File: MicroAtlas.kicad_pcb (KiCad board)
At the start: 4 copper layers, 20 x 32.8 mm, 38 parts, among them J1 TAGCONNECT, J2 Conn_01x02, J3 Conn_01x04_MountingPin, J4 SMA_Edgelaunch, J5 UFL, U1 NEO-F9P, U2 RAK3172-xx-43-SM-xI, U3 TPS7A2033PDBVR, U4 W25Q32JVZP, U5 TPS2116DRL, U6 LSM6DSV320XTR

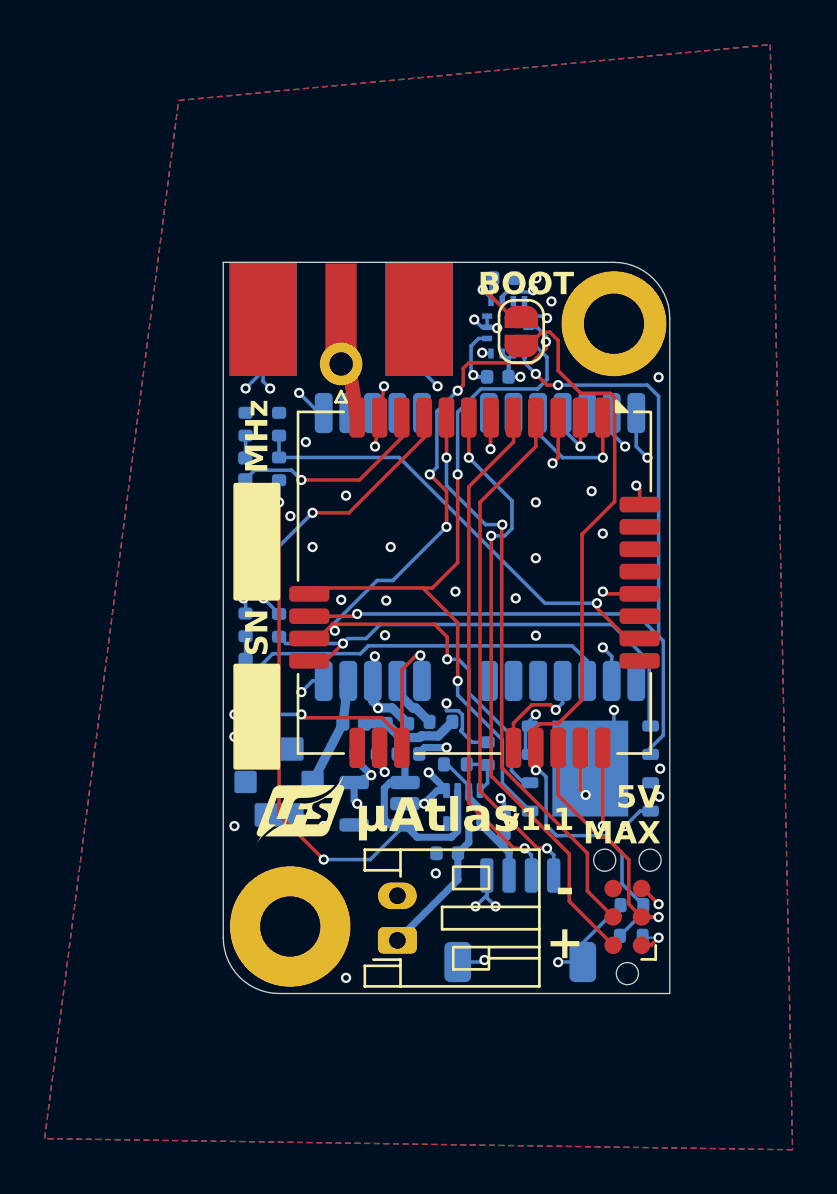
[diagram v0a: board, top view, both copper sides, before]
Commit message: prod v2.0
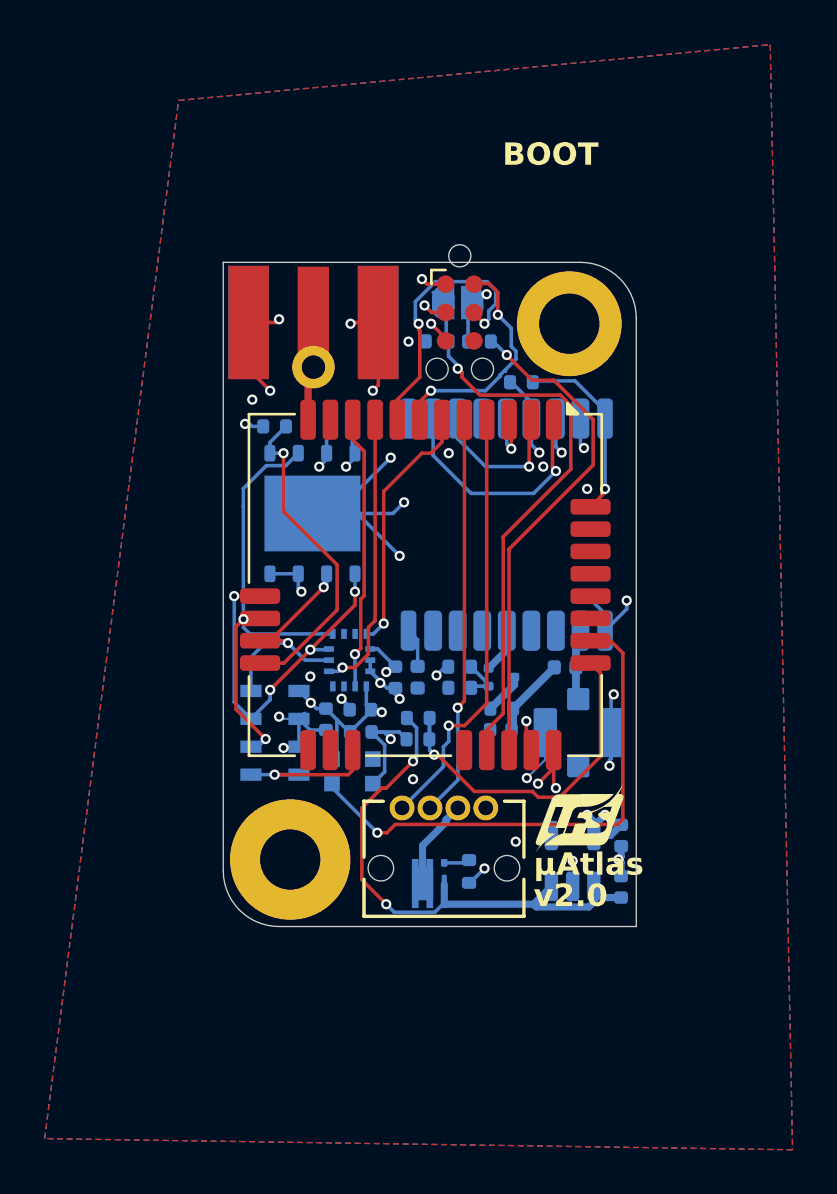
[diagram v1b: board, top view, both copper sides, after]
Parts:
- removed C46: 0.1uF, Capacitor_SMD:C_0402_1005Metric
- removed D7, D8: PPS, LED_SMD:LED_0402_1005Metric
- removed J3: Conn_01x04_MountingPin, Connector_JST:JST_SH_SM04B-SRSS-TB_1x04-1MP_P1.00mm_Horizontal
- removed R56, R57: 1k, Resistor_SMD:R_0402_1005Metric
- removed R58: 36k, Resistor_SMD:R_0402_1005Metric
- removed R59: 10k, Resistor_SMD:R_0402_1005Metric
- removed U4: W25Q32JVZP, Package_SON:WSON-8-1EP_6x5mm_P1.27mm_EP3.4x4.3mm
- added C48: 0.1uF, Capacitor_SMD:C_0402_1005Metric, B.Cu at (76.2, 52.8)
- added C51: 0.1uF, Capacitor_SMD:C_0402_1005Metric, B.Cu at (73.8, 41.6)
- added D1: WS2812B-2020, LED_SMD:LED_WS2812B-2020_PLCC4_2.0x2.0mm, B.Cu at (74.3, 57.0)
- added Q1: NTK3139PT1G, Package_TO_SOT_SMD:SOT-723, B.Cu at (81.0, 52.8)
- added Q2: SiA449DJ, Package_TO_SOT_SMD:Vishay_PowerPAK_SC70-6L_Single, B.Cu at (77.8, 62.1)
- added R49: 100k, Resistor_SMD:R_0402_1005Metric, B.Cu at (79.5, 61.5)
- added R60: 10k, Resistor_SMD:R_0402_1005Metric, B.Cu at (79.1, 52.4)
- added U7: LSM6DSV320XTR, PCM_SparkFun-Sensor:ST_LGA-14L_2.5x3.0mm_P0.5mm_4x3, B.Cu at (74.2, 52.1)
- C45: value 1uF -> 2.2uF
- C49, C50: value 4.7uF -> 0.1uF
- J2: value Conn_01x02 -> Conn_01x04_Socket; footprint Connector_JST:JST_PH_S2B-PH-K_1x02_P2.00mm_Horizontal -> FCU2025Lib:CONN_2200980000-SD_04P_MOL
- JP1: moved to B.Cu
- R55: value 1k -> 100R
- U1: value NEO-F9P -> W25Q32JVZP; footprint RF_GPS:ublox_NEO -> Package_SON:WSON-8-1EP_6x5mm_P1.27mm_EP3.4x4.3mm
- U3: value TPS7A2033PDBVR -> TPS7E7233
- U5: value TPS2116DRL -> MS5611-01BA; footprint Package_TO_SOT_SMD:SOT-583-8 -> Package_LGA:LGA-8_3x5mm_P1.25mm
- U6: value LSM6DSV320XTR -> MAX-M11S; footprint PCM_SparkFun-Sensor:ST_LGA-14L_2.5x3.0mm_P0.5mm_4x3 -> RF_GPS:ublox_MAX
- moved J1 28.1 mm to (79.1, 36.5), turned to -90 degrees
- moved R4 27.5 mm to (80.0, 37.8), turned to 180 degrees
- moved R3 26.7 mm to (78.1, 37.8)
- moved C47 20.4 mm to (74.6, 54.3), turned to 0 degrees
- moved R5 18.8 mm to (81.9, 39.6)
- moved R2 15.4 mm to (77.2, 55.6), turned to 180 degrees
- moved J5 13.6 mm to (84.4, 55.3), turned to 0 degrees
- moved R1 12.8 mm to (77.2, 54.7), turned to 0 degrees
- moved G*** 12.5 mm to (84.4, 59.2)
- moved C45 12.0 mm to (86.3, 59.9), turned to 90 degrees
- moved C44 11.2 mm to (86.3, 62.2), turned to -90 degrees
- moved R55 10.00 mm to (79.1, 53.3), turned to 0 degrees
- moved FB2 9.80 mm to (83.8, 52.4), turned to 180 degrees
- moved U5 9.07 mm to (70.8, 55.3), turned to 180 degrees
- moved U3 9.02 mm to (84.1, 61.1), turned to 90 degrees
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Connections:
- C49 pad 2: Net-(J2-Pin_1) -> +3V3
- C50 pad 2: +5V -> +3V3
- D6 pad 1: Net-(D6-K) -> GND
- J2 pad 1: Net-(J2-Pin_1) -> /TX
- J2 pad 2: GND -> /RX
- R54 pad 1: Net-(U1-VCC_RF) -> Net-(Q1-D)
- R55 pad 1: GND -> /EXT_ANT
- R55 pad 2: Net-(D6-K) -> Net-(Q1-G)
- U1 pad 1: unconnected-(U1-~{SAFEBOOT}-Pad1) -> /CS_FLASH
- U1 pad 2: +3V3 -> /MISO
- U1 pad 3: Net-(D6-A) -> +3V3
- U1 pad 4: /GPS_INT -> GND
- U1 pad 5: unconnected-(U1-USB_DM-Pad5) -> /MOSI
- U1 pad 6: unconnected-(U1-USB_DP-Pad6) -> /SCK
- U1 pad 7: unconnected-(U1-VDD_USB-Pad7) -> +3V3
- U1 pad 8: /GPS_NRST -> +3V3
- U1 pad 9: Net-(U1-VCC_RF) -> GND
- U2 pad 10: /P2 -> /IMU_INT2
- U2 pad 19: /GPS_NRST -> /CS_BARO
- U2 pad 20: /GPS_INT -> unconnected-(U2-PA9-Pad20)
- U2 pad 25: unconnected-(U2-PA10/PIN_A3-Pad25) -> /VDIV
- U2 pad 26: /VDIV -> /RGB
- U2 pad 3: /IMU_INT2 -> /GPS_INT
- U2 pad 32: /IMU_CS -> /GPS_NRST
- U2 pad 9: /P1 -> /IMU_CS
- U5 pad 1: GND -> +3V3
- U5 pad 2: V_LIPO -> GND
- U5 pad 3: +5V -> GND
- U5 pad 4: Net-(U5-PR1) -> /CS_BARO
- U5 pad 5: +5V -> /CS_BARO
- U5 pad 6: Net-(J2-Pin_1) -> /MISO
- U5 pad 7: V_LIPO -> /MOSI
- U5 pad 8: unconnected-(U5-ST-Pad8) -> /SCK
- U6 pad 1: /MISO -> GND
- U6 pad 10: unconnected-(U6-OCS_Aux-Pad10) -> GND
- U6 pad 11: unconnected-(U6-SDO_Aux-Pad11) -> Net-(J5-In)
- U6 pad 12: /IMU_CS -> GND
- U6 pad 13: /SCK -> unconnected-(U6-LNA_EN-Pad13)
- U6 pad 14: /MOSI -> Net-(Q1-S)
- U6 pad 2: GND -> /GPS_RX
- U6 pad 3: GND -> /GPS_TX
- U6 pad 4: /IMU_INT1 -> /TP
- U6 pad 5: +3V3 -> /GPS_INT
- U6 pad 6: GND -> +3V3
- U6 pad 7: GND -> +3V3
- U6 pad 9: /IMU_INT2 -> /GPS_NRST
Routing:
- net /SCK: track 36.0 -> 11.4 mm, vias 6 -> 2
- net /RGB: track 0.00 -> 23.4 mm, vias 0 -> 1
- net /MISO: track 39.6 -> 21.1 mm, vias 3 -> 2
- net /SWDIO: track 27.4 -> 10.5 mm
- net /MOSI: track 32.5 -> 16.2 mm, vias 2 -> 4
- net /NRST: track 12.1 -> 28.0 mm, vias 1 -> 2
- net Net-(D6-A): track 17.1 -> 2.03 mm
- net /SWCLK: track 25.9 -> 12.3 mm
- net /P1: track 11.5 -> 0.00 mm, vias 1 -> 0
- net /P2: track 9.06 -> 0.00 mm, vias 1 -> 0
- net /BOOT: track 34.9 -> 26.8 mm
- net /CS_FLASH: track 22.6 -> 14.6 mm
- net +3V3: track 25.6 -> 32.7 mm, vias 12 -> 15
- net V_LIPO: track 31.5 -> 24.8 mm
- net /CS_BARO: track 0.00 -> 6.63 mm, vias 0 -> 1
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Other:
- board size 20 x 32.8 mm -> 18.5 x 29.8 mm
- board text added: "G V R T"
- board text added: "v2.0"
- board text removed: "- +"
- board text removed: "5V MAX"
- board text removed: "MHz"
- board text removed: "SN"
- board text removed: "TR5G"
- board text removed: "UART"
- board text removed: "v1.1"
